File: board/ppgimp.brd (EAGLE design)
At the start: 160 x 100 mm, 20 parts, among them J1 VDD, J2 GND, J3 SPI, J4 I_Test, J5 R_test, J6 SDA, U1 LM334Z/NOPB, U2 AD8400ARZ1, U3 AD8400ARZ10, U4 AD8400ARZ10, U5 AD5933YRSZ, U6 ADG1609

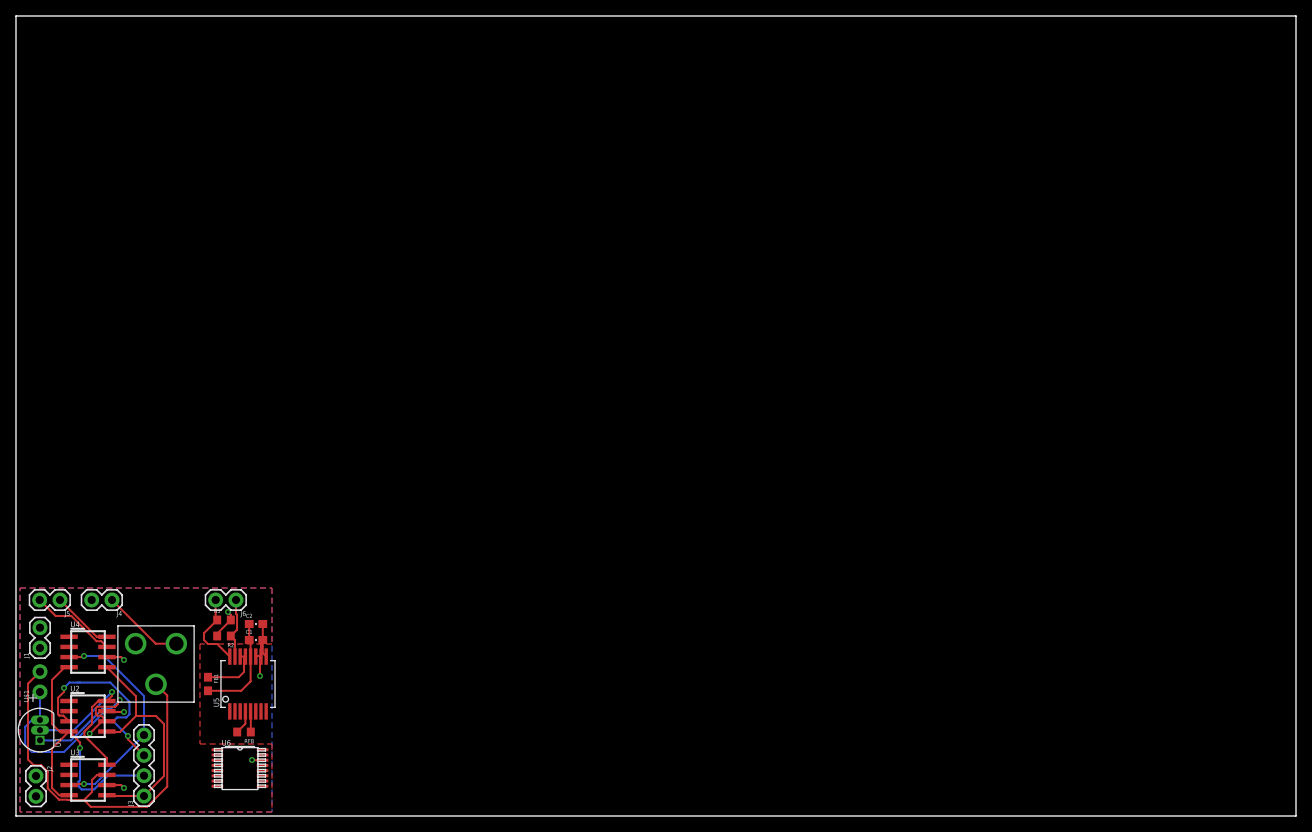
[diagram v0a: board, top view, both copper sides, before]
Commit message: finish up test board
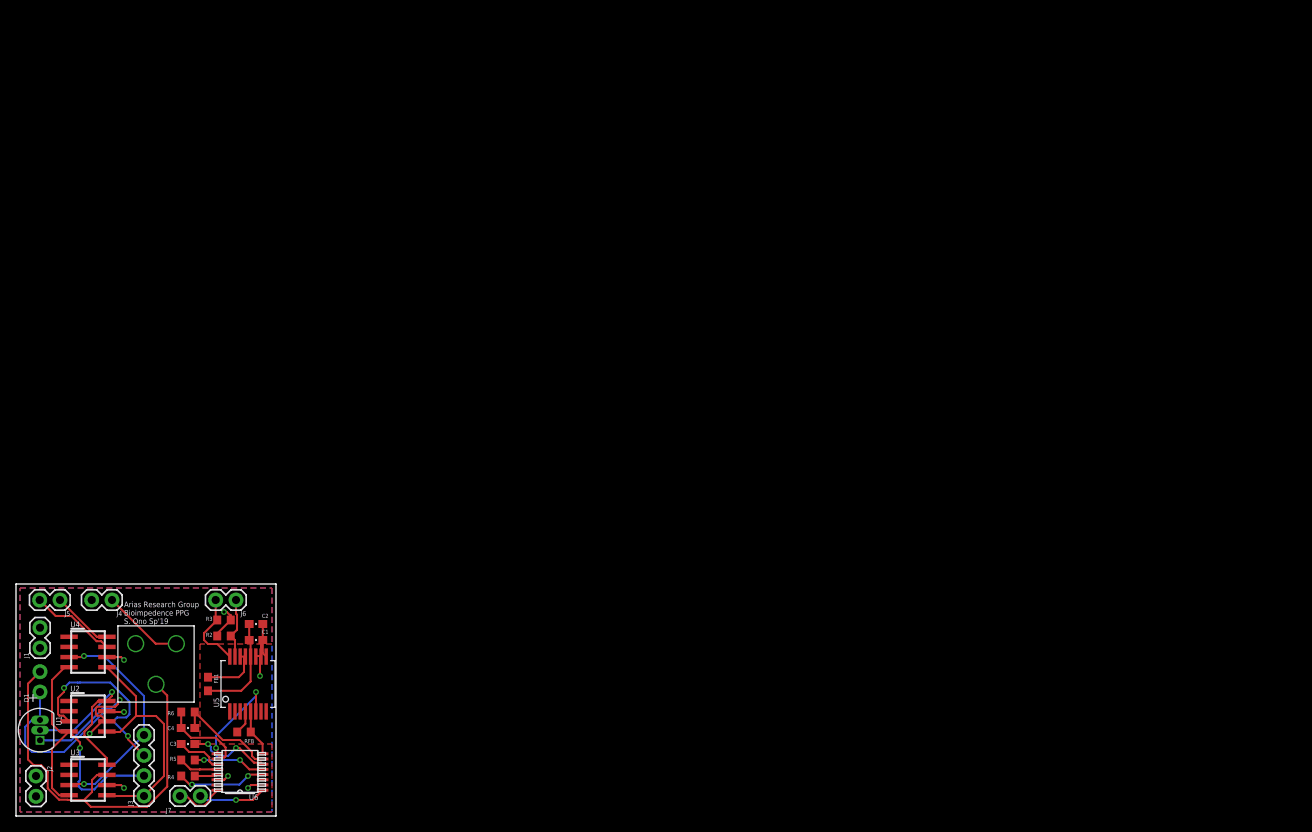
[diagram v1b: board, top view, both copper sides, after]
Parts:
- added C3, C4: 1uF, scono:0603-CAP
- added J7: SEL, scono:1X02
- added R4: 510K, scono:R0603
- added R5: 200K, scono:R0603
- added R6: 100K, scono:R0603
- R2, R3: value (none) -> 10K
- moved U6 0.50 mm to (28.0, 5.50), turned to 180 degrees
- renumbered U$1 to D1
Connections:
- new net N$10: C3.2, U6.11
- new net N$11: C4.1, R6.1, U6.7
- new net N$12: C4.2, R6.2, U6.10
- new net N$3: J7.1, U6.16
- new net N$4: J7.2, U6.1
- new net N$5: R4.2, U6.4
- new net N$6: R4.1, U6.13
- new net N$7: R5.2, U6.5
- new net N$8: R5.1, U6.12
- new net N$9: C3.1, U6.6
- net GND: now also U6.15, U6.3
- net VDD: now also U6.2
- net VIN: now also U6.8
- net VOUT: now also U6.9
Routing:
- net N$11: track 0.00 -> 13.2 mm
- net VOUT: track 0.00 -> 12.3 mm, vias 0 -> 2
- net N$5: track 0.00 -> 11.1 mm, vias 0 -> 2
- net N$12: track 0.00 -> 10.8 mm
- net N$9: track 0.00 -> 10.6 mm, vias 0 -> 2
- net N$7: track 0.00 -> 8.96 mm, vias 0 -> 2
- net N$4: track 0.00 -> 8.49 mm, vias 0 -> 1
- net N$3: track 0.00 -> 6.17 mm
- net N$10: track 0.00 -> 5.87 mm
- net N$8: track 0.00 -> 5.02 mm
- net VIN: track 2.58 -> 5.92 mm
- net N$6: track 0.00 -> 2.90 mm
- net VDD: track 40.7 -> 43.5 mm, vias 7 -> 8
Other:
- board size 160 x 100 mm -> 32.5 x 29 mm
- board text added: "Arias Research Group Bioimpedence PPG S. Ono Sp'19"
